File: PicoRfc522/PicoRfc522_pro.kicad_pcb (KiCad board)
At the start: 2 copper layers, 100 x 90 mm, 19 parts, among them J1 5V sel, J2 Grove 2mm, J3 Screw_Terminal_01x04, J4 Screw_Terminal_01x02, J5 IDC1, J6 IDC1, J7 IDC1, J8 IDC1, Q1 DMG2305UX-7, SW1 SW_Push, U1 AMS1117-3.3, U2 AMS1117-5.0, U3 Pico_RaspberryPico

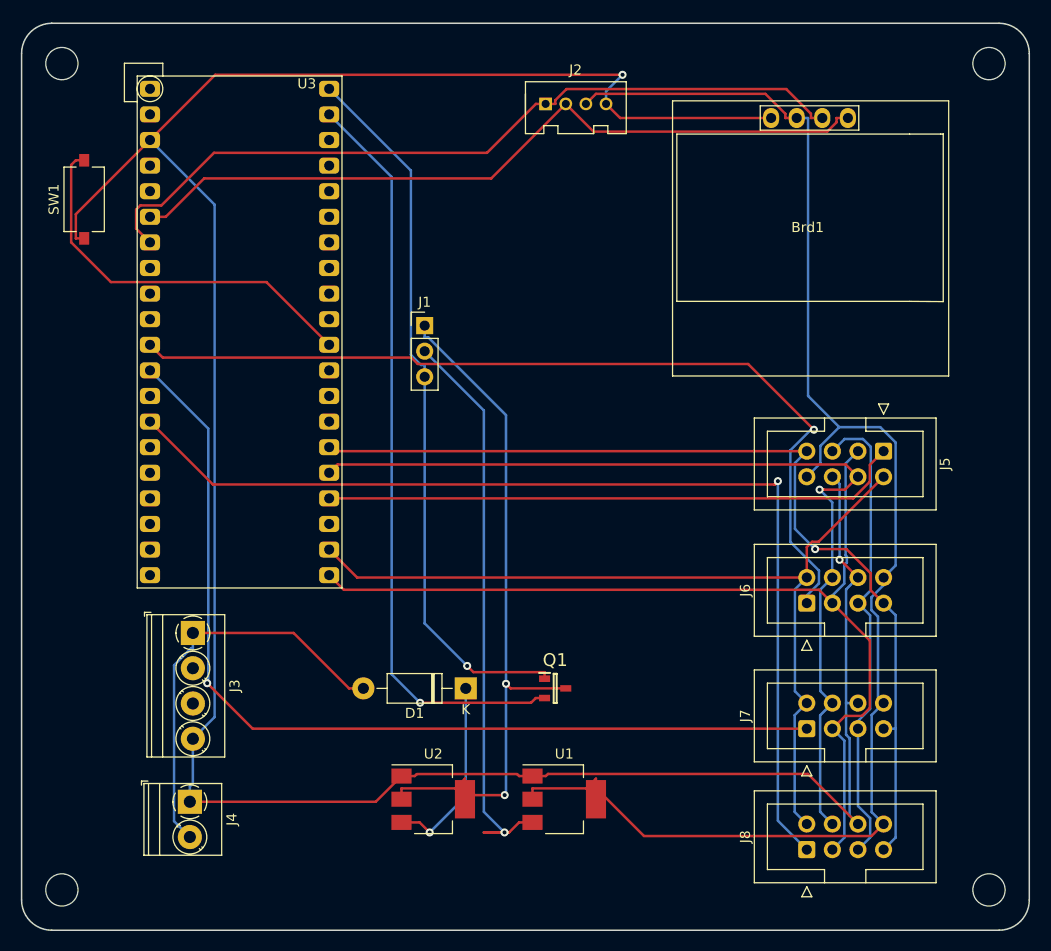
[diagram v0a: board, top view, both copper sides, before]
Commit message: 07/09/25 21:50 Titan.local
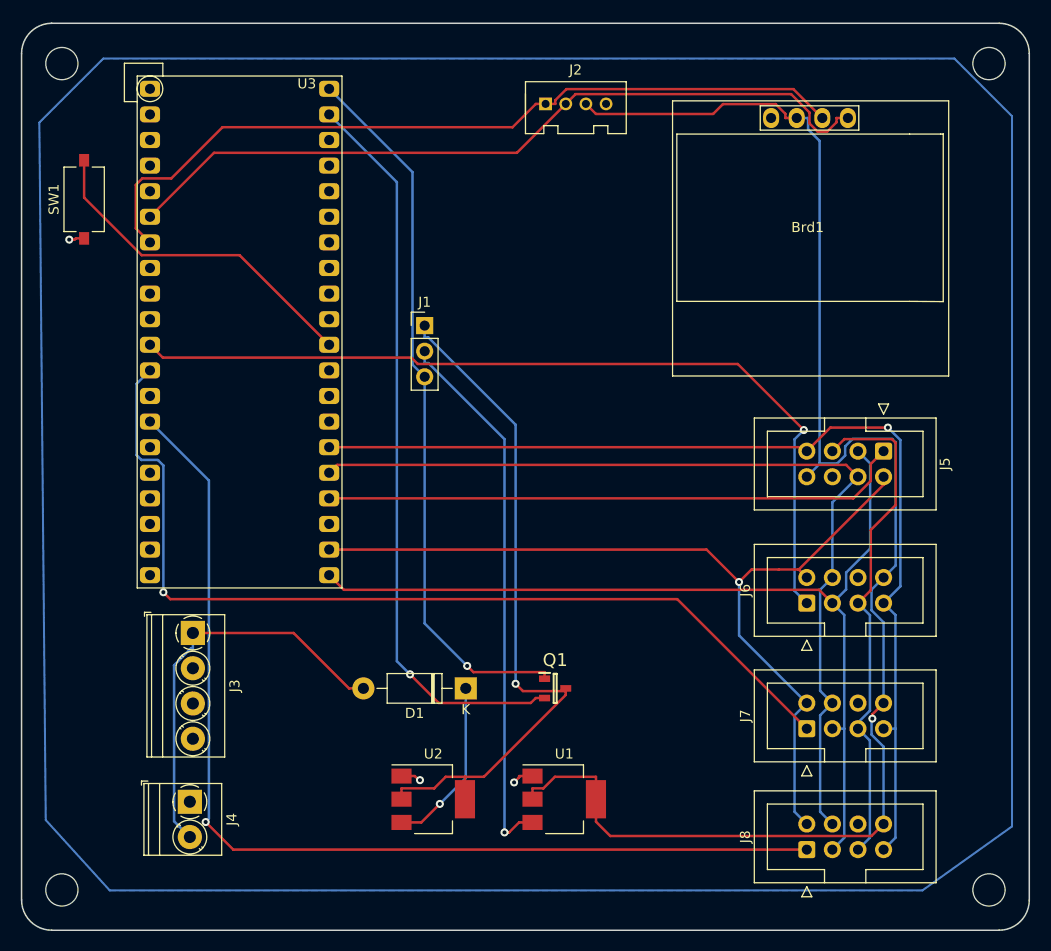
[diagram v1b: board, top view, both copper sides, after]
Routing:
- net /GND: track 260.4 -> 5.70 mm, vias 2 -> 3
- net /5Vopt: track 62.4 -> 54.4 mm
- net /RST: track 95.2 -> 101.8 mm
- net Net-(U3-RUN): track 39.0 -> 34.1 mm
- net /MISO: track 95.0 -> 90.8 mm, vias 1 -> 0
- net /IRQ: track 47.1 -> 50.8 mm
- net /CS2: track 89.5 -> 86.4 mm
- net /3V3: track 149.4 -> 151.8 mm, vias 0 -> 1
- net /MOSI: track 96.8 -> 94.8 mm
- net /12V: track 19.0 -> 17.1 mm
- net /CS4: track 104.6 -> 103.1 mm
- net /SCK: track 88.5 -> 90.1 mm, vias 0 -> 1
- net /SDA: track 75.8 -> 77.3 mm
- net /5V: track 70.3 -> 68.9 mm, vias 2 -> 1
- net /SCL: track 78.5 -> 79.7 mm
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- added copper zone on B.Cu, net /GND

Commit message: 07/09/25 22:20 Titan.local
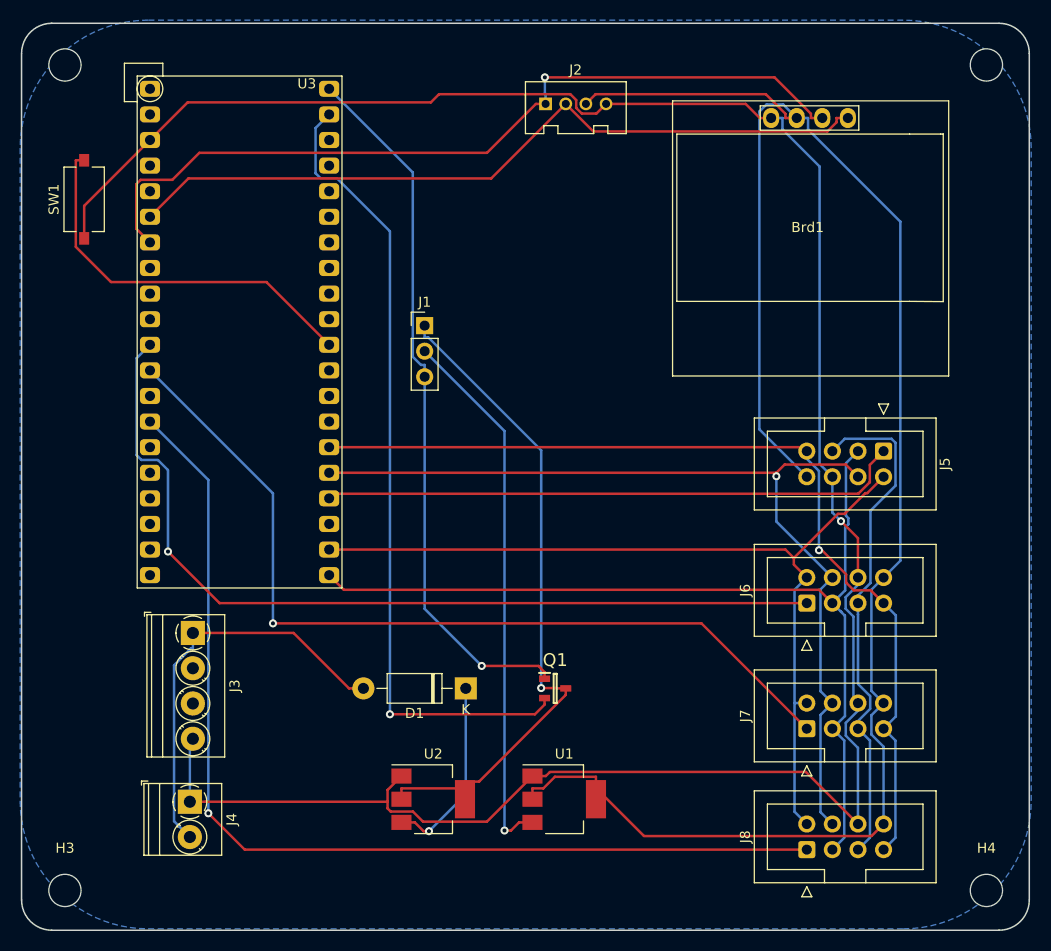
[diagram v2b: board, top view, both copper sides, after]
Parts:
- H1, H2, H3, H4: value MountingHole -> MountingHole_3.2mm_M3; footprint MountingHole:MountingHole_3.2mm_M3_DIN965 -> MountingHole:MountingHole_3.2mm_M3
- moved H1 0.33 mm to (154.3, 64.1)
- moved H3 0.31 mm to (154.3, 146.1)
- moved H2 0.29 mm to (245.7, 64.1)
- moved H4 0.26 mm to (245.7, 146.1)
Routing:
- net /GND: track 5.70 -> 235.7 mm, vias 3 -> 1
- net /3V3: track 151.8 -> 184.0 mm, vias 1 -> 0
- net /RST: track 101.8 -> 93.4 mm
- net /VSYS: track 73.6 -> 80.5 mm
- net /CS3: track 94.1 -> 87.5 mm
- net Net-(U3-RUN): track 34.1 -> 38.6 mm
- net /SCL: track 79.7 -> 82.4 mm, vias 0 -> 1
- net /CS2: track 86.4 -> 88.8 mm
- net /SCK: track 90.1 -> 87.9 mm, vias 1 -> 0
- net /5V: track 68.9 -> 67.0 mm
- net /12V: track 17.1 -> 18.8 mm
- net /MISO: track 90.8 -> 92.4 mm, vias 0 -> 1
- net /SDA: track 77.3 -> 75.8 mm
- net /MOSI: track 94.8 -> 93.9 mm
- net /CS4: track 103.1 -> 102.1 mm
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- added copper zone on B.Cu, net (none)
- removed copper zone on B.Cu, net /GND
